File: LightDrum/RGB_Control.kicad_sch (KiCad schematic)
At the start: 0 parts

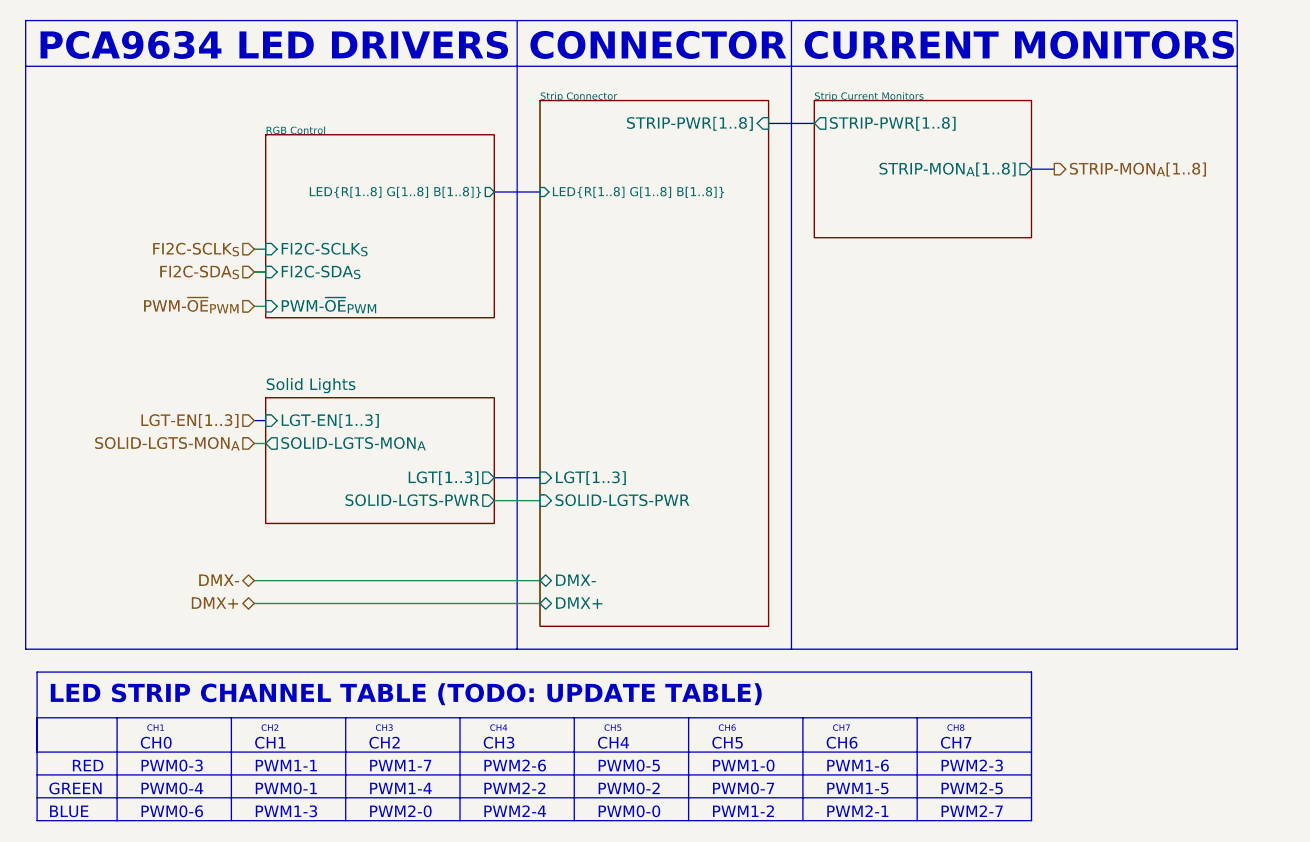
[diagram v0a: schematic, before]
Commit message: (WIP) REV12 Testing and firmware dev
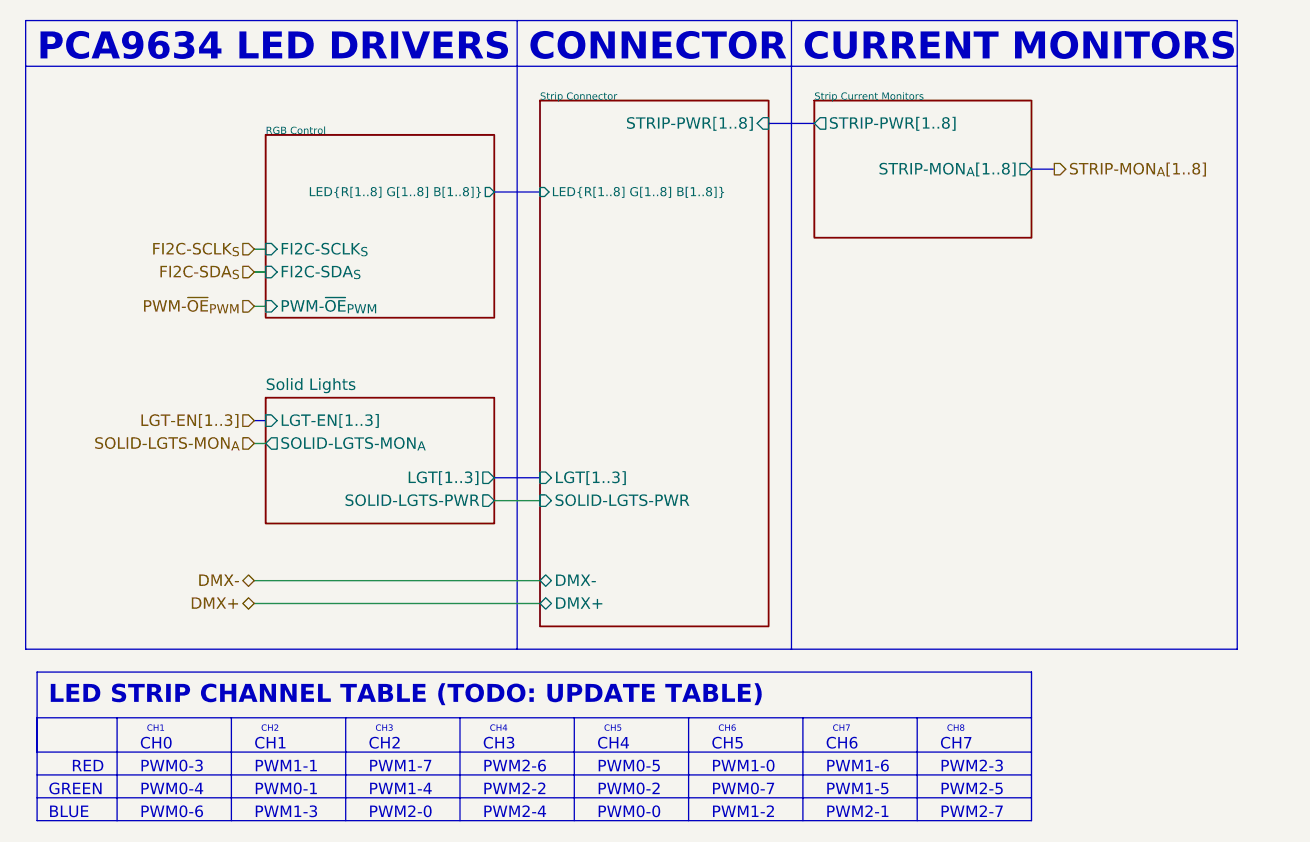
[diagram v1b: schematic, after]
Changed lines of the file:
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@@
   (title_block
     (title "LightDrum")
-    (rev "REV11")
+    (rev "REV13")
     (company "Daxxn Industries")
   )
@@
   )
   (sheet (at 69.85 21.59) (size 25.4 58.42)
-    (stroke (width 0.1524) (type solid))
+    (stroke (width 0.2) (type solid))
     (fill (color 0 0 0 0.0000))
     (property "Sheetname" "Strip Connector" (at 69.85 21.59 0)
@@
   )
   (sheet (at 39.37 25.4) (size 25.4 20.32)
-    (stroke (width 0.1524) (type solid))
+    (stroke (width 0.2) (type solid))
     (fill (color 0 0 0 0.0000))
     (property "Sheetname" "RGB Control" (at 39.37 25.4 0)
@@
   )
   (sheet (at 100.33 21.59) (size 24.13 15.24)
-    (stroke (width 0.1524) (type solid))
+    (stroke (width 0.2) (type solid))
     (fill (color 0 0 0 0.0000))
     (property "Sheetname" "Strip Current Monitors" (at 100.33 21.59 0)
@@
   )
   (sheet (at 39.37 54.61) (size 25.4 13.97) (fields_autoplaced)
-    (stroke (width 0.1524) (type solid))
+    (stroke (width 0.2) (type solid))
     (fill (color 0 0 0 0.0000))
     (property "Sheetname" "Solid Lights" (at 39.37 53.8984 0)
